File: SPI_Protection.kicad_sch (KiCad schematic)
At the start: 5 parts, among them Q14 MMBT2907

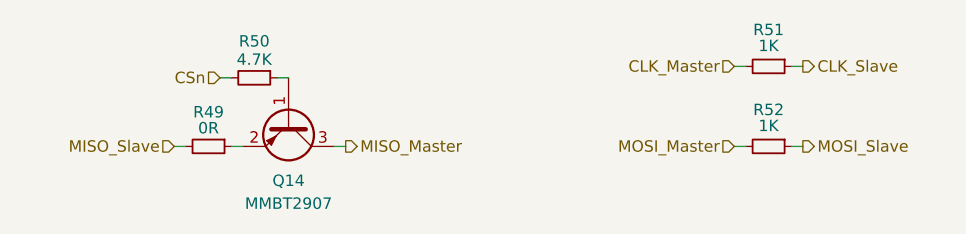
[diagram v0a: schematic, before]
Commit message: v3 partial schematic updates
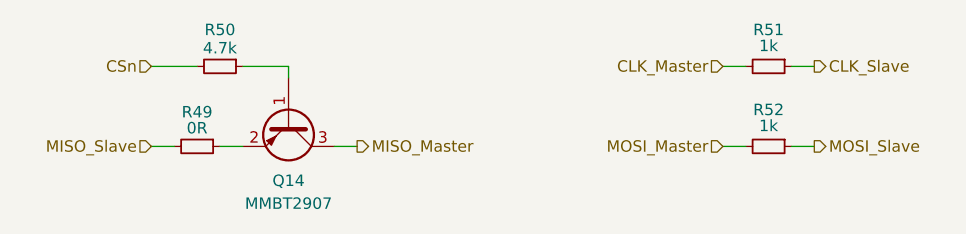
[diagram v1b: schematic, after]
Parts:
- R50: value 4.7K -> 4.7k
- R51, R52: value 1K -> 1k
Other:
- moved on the sheet: R49, R50
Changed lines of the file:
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@@
 	(wire
 		(pts
-			(xy 176.53 91.44) (xy 177.8 91.44)
-		)
-		(stroke
-			(width 0)
-			(type default)
-		)
-	)
-	(wire
-		(pts
-			(xy 176.53 100.33) (xy 177.8 100.33)
-		)
-		(stroke
-			(width 0)
-			(type default)
-		)
-	)
-	(wire
-		(pts
-			(xy 114.3 100.33) (xy 115.57 100.33)
-		)
-		(stroke
-			(width 0)
-			(type default)
-		)
-	)
-	(wire
-		(pts
-			(xy 127 100.33) (xy 125.73 100.33)
-		)
-		(stroke
-			(width 0)
-			(type default)
-		)
-	)
-	(wire
-		(pts
-			(xy 107.95 100.33) (xy 109.22 100.33)
-		)
-		(stroke
-			(width 0)
-			(type default)
-		)
-	)
-	(wire
-		(pts
-			(xy 170.18 91.44) (xy 171.45 91.44)
-		)
-		(stroke
-			(width 0)
-			(type default)
-		)
-	)
-	(wire
-		(pts
-			(xy 113.03 92.71) (xy 114.3 92.71)
-		)
-		(stroke
-			(width 0)
-			(type default)
-		)
-	)
-	(wire
-		(pts
-			(xy 119.38 92.71) (xy 120.65 92.71)
-		)
-		(stroke
-			(width 0)
-			(type default)
-		)
-	)
-	(wire
-		(pts
-			(xy 170.18 100.33) (xy 171.45 100.33)
+			(xy 176.53 91.44) (xy 179.07 91.44)
+		)
+		(stroke
+			(width 0)
+			(type default)
+		)
+	)
+	(wire
+		(pts
+			(xy 176.53 100.33) (xy 179.07 100.33)
+		)
+		(stroke
+			(width 0)
+			(type default)
+		)
+	)
+	(wire
+		(pts
+			(xy 113.03 100.33) (xy 115.57 100.33)
+		)
+		(stroke
+			(width 0)
+			(type default)
+		)
+	)
+	(wire
+		(pts
+			(xy 128.27 100.33) (xy 125.73 100.33)
+		)
+		(stroke
+			(width 0)
+			(type default)
+		)
+	)
+	(wire
+		(pts
+			(xy 105.41 100.33) (xy 107.95 100.33)
+		)
+		(stroke
+			(width 0)
+			(type default)
+		)
+	)
+	(wire
+		(pts
+			(xy 168.91 91.44) (xy 171.45 91.44)
+		)
+		(stroke
+			(width 0)
+			(type default)
+		)
+	)
+	(wire
+		(pts
+			(xy 120.65 91.44) (xy 120.65 92.71)
+		)
+		(stroke
+			(width 0)
+			(type default)
+		)
+	)
+	(wire
+		(pts
+			(xy 105.41 91.44) (xy 110.49 91.44)
+		)
+		(stroke
+			(width 0)
+			(type default)
+		)
+	)
+	(wire
+		(pts
+			(xy 115.57 91.44) (xy 120.65 91.44)
+		)
+		(stroke
+			(width 0)
+			(type default)
+		)
+	)
+	(wire
+		(pts
+			(xy 168.91 100.33) (xy 171.45 100.33)
 		)
 		(stroke
@@
 	(hierarchical_label "MOSI_Master"
 		(shape input)
-		(at 170.18 100.33 180)
+		(at 168.91 100.33 180)
 		(fields_autoplaced yes)
 		(effects
@@
 	(hierarchical_label "MOSI_Slave"
 		(shape output)
-		(at 177.8 100.33 0)
+		(at 179.07 100.33 0)
 		(fields_autoplaced yes)
 		(effects
@@
 	(hierarchical_label "CLK_Slave"
 		(shape output)
-		(at 177.8 91.44 0)
+		(at 179.07 91.44 0)
 		(fields_autoplaced yes)
 		(effects
@@
 	(hierarchical_label "MISO_Slave"
 		(shape input)
-		(at 107.95 100.33 180)
+		(at 105.41 100.33 180)
 		(fields_autoplaced yes)
 		(effects
@@
 	(hierarchical_label "CSn"
 		(shape input)
-		(at 113.03 92.71 180)
+		(at 105.41 91.44 180)
 		(fields_autoplaced yes)
 		(effects
@@
 	(hierarchical_label "MISO_Master"
 		(shape output)
-		(at 127 100.33 0)
+		(at 128.27 100.33 0)
 		(fields_autoplaced yes)
 		(effects
@@
 	(hierarchical_label "CLK_Master"
 		(shape input)
-		(at 170.18 91.44 180)
+		(at 168.91 91.44 180)
 		(fields_autoplaced yes)
 		(effects
@@
 	(symbol
 		(lib_id "Device:R_Small")
-		(at 116.84 92.71 270)
+		(at 113.03 91.44 270)
 		(unit 1)
 		(exclude_from_sim no)
@@
 		(dnp no)
 		(property "Reference" "R50"
-			(at 116.84 88.646 90)
-			(effects
-				(font
-					(size 1.27 1.27)
-				)
-			)
-		)
-		(property "Value" "4.7K"
-			(at 116.84 90.678 90)
+			(at 113.03 87.376 90)
+			(effects
+				(font
+					(size 1.27 1.27)
+				)
+			)
+		)
+		(property "Value" "4.7k"
+			(at 113.03 89.408 90)
 			(effects
 				(font
@@
 		)
 		(property "Footprint" "Resistor_SMD:R_0603_1608Metric"
-			(at 116.84 92.71 0)
+			(at 113.03 91.44 0)
 			(effects
 				(font
@@
 		)
 		(property "Datasheet" "~"
-			(at 116.84 92.71 0)
+			(at 113.03 91.44 0)
 			(effects
 				(font
@@
 		)
 		(property "Description" "Resistor, small symbol"
-			(at 116.84 92.71 0)
+			(at 113.03 91.44 0)
 			(effects
 				(font
@@
 			)
 		)
-		(property "Value" "1K"
+		(property "Value" "1k"
 			(at 173.99 98.044 90)
 			(effects
@@
 			)
 		)
-		(property "Value" "1K"
+		(property "Value" "1k"
 			(at 173.99 89.154 90)
 			(effects
@@
 	(symbol
 		(lib_id "Device:R_Small")
-		(at 111.76 100.33 270)
+		(at 110.49 100.33 270)
 		(unit 1)
 		(exclude_from_sim no)
@@
 		(dnp no)
 		(property "Reference" "R49"
-			(at 111.76 96.52 90)
+			(at 110.49 96.52 90)
 			(effects
 				(font
@@
 		)
 		(property "Value" "0R"
-			(at 111.76 98.298 90)
+			(at 110.49 98.298 90)
 			(effects
 				(font
@@
 		)
 		(property "Footprint" "Resistor_SMD:R_0603_1608Metric"
-			(at 111.76 100.33 0)
+			(at 110.49 100.33 0)
 			(effects
 				(font
@@
 		)
 		(property "Datasheet" "~"
-			(at 111.76 100.33 0)
+			(at 110.49 100.33 0)
 			(effects
 				(font
@@
 		)
 		(property "Description" "Resistor, small symbol"
-			(at 111.76 100.33 0)
-			(effects
-				(font
+			(at 110.49 100.33 0)
+			(effects
+				(font
